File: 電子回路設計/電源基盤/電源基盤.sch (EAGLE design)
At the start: 59 parts, among them IC1 FDS4935A, IC2 NJM7805FA-I, SW1 SS-12D01-VG4, T1 TLP291, T2 TLP291, T3 TJ60S04M3L, T4 TLP291, T5 IRLML6344TRPBF

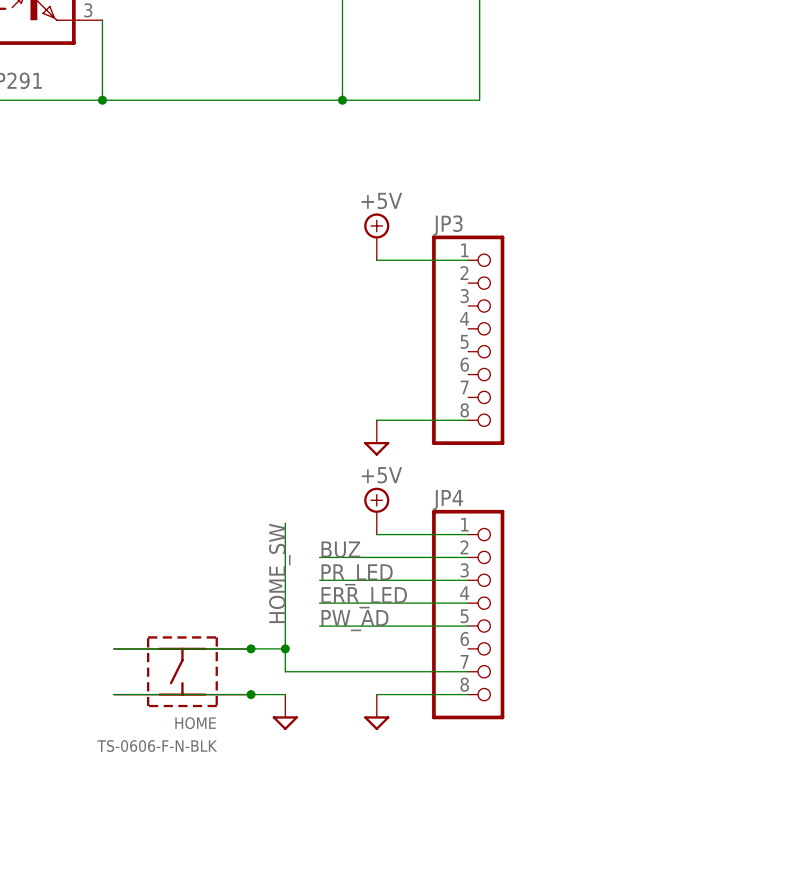
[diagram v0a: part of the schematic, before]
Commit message: point : circuit desgine comp
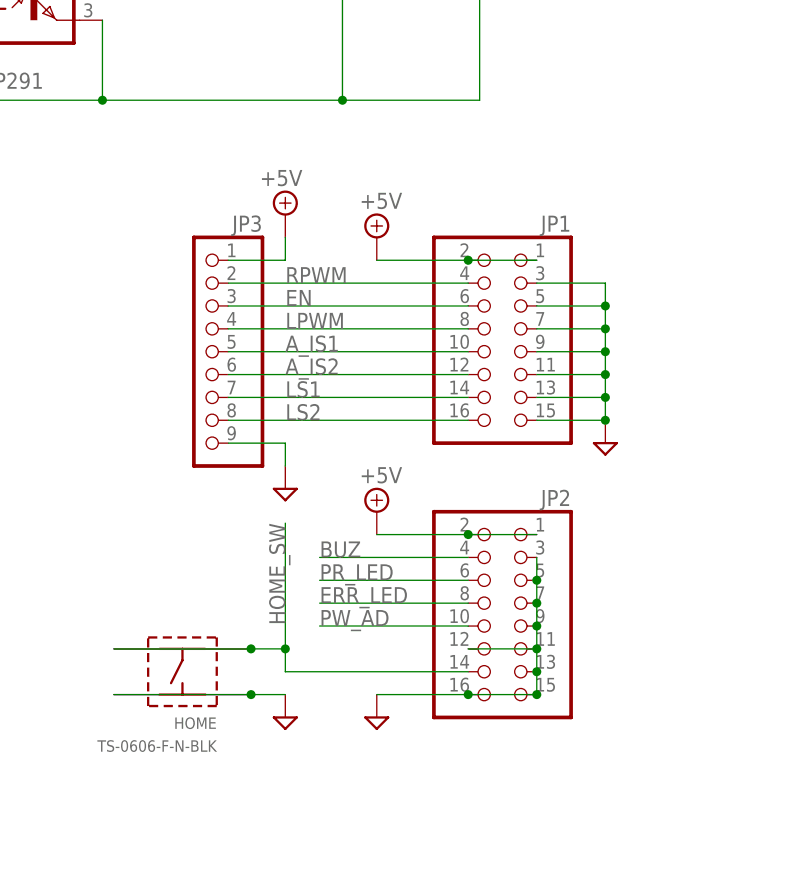
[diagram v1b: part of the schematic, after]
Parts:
- removed JP4: (no value), pinhead:PINHD-1X8
- added JP1, JP2: (no value), pinhead:PINHD-2X8
- JP3: device pinhead:PINHD-1X8 -> pinhead:PINHD-1X9
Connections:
- new net A_IS1: JP1.10, JP3.5
- new net A_IS2: JP1.12, JP3.6
- new net EN: JP1.6, JP3.3
- new net LPWM: JP1.8, JP3.4
- new net LS1: JP1.14, JP3.7
- new net LS2: JP1.16, JP3.8
- new net RPWM: JP1.4, JP3.2
- net +5V: now also JP1.1, JP1.2, JP2.1, JP2.2; no longer JP4.1
- net BUZ: now also JP2.4; no longer JP4.2
- net ERR_LED: now also JP2.6; no longer JP4.3
- net GND: now also JP1.11, JP1.13, JP1.15, JP1.3, JP1.5, JP1.7, JP1.9, JP2.11, JP2.12, JP2.13, JP2.15, JP2.16, JP2.3, JP2.5, JP2.7, JP2.9, JP3.9; no longer JP3.8, JP4.8
- net HOME_SW: now also JP2.14; no longer JP4.7
- net PR_LED: now also JP2.8; no longer JP4.4
- net PW_AD: now also JP2.10; no longer JP4.5
